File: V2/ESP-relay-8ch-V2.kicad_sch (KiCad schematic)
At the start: 143 parts, among them J1 +24VDC, J10 OUT8, J2 INPUTS, J3 OUT1, J4 OUT2, J5 OUT3, J6 OUT4, J7 OUT5, J8 OUT6, J9 OUT7, K1 G5PZ-1A, K2 G5PZ-1A, K3 G5PZ-1A, K4 G5PZ-1A, K5 G5PZ-1A, K6 G5PZ-1A, K7 G5PZ-1A, K8 G5PZ-1A, Q1 MMBT2222A/SOT-23-3, Q2 MMBT2222A/SOT-23-3, Q3 MMBT2222A/SOT-23-3, Q4 MMBT2222A/SOT-23-3, Q5 MMBT2222A/SOT-23-3, Q6 MMBT2222A/SOT-23-3, Q7 MMBT2222A/SOT-23-3, Q8 MMBT2222A/SOT-23-3, U1 SY8089A1AAC, U10 TX4138, U11 Olimex_ESP32-POE, U2 LTV-817S, U3 LTV-817S, U4 LTV-817S, U5 LTV-817S, U6 LTV-817S, U7 LTV-817S, U8 LTV-817S, U9 LTV-817S

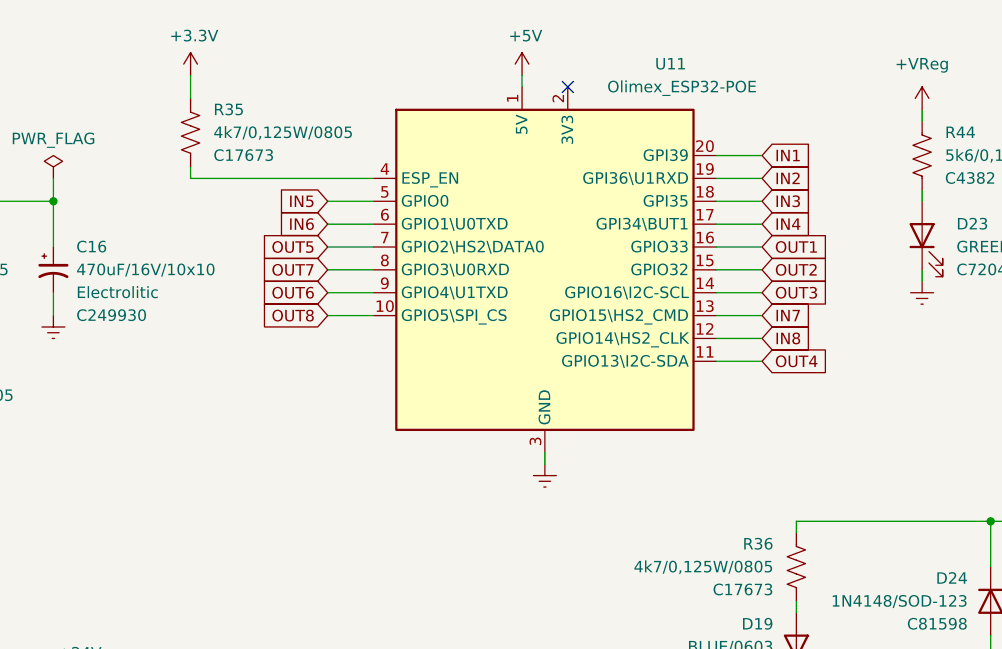
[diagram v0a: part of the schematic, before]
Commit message: Dev
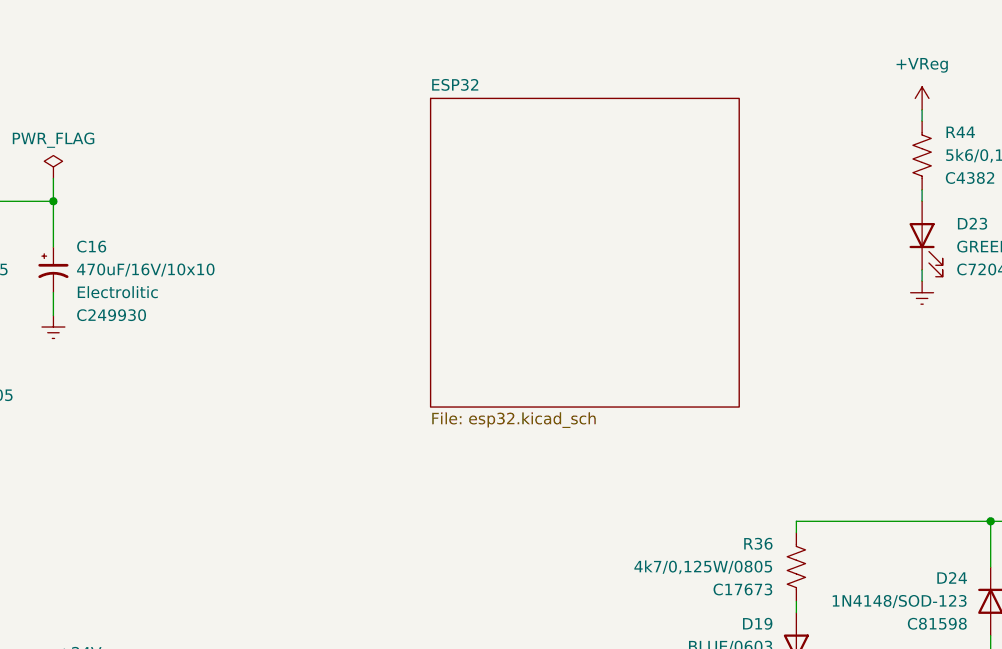
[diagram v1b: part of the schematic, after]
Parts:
- removed R35: 4k7/0,125W/0805, Tales:R_0805_2012Metric, symbol Device:R_US
- removed U11: Olimex_ESP32-POE, Tales:Olimex_ESP32-POE_Pads, symbol Tales:Olimex_ESP32-POE
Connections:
- no-connect marks 3 -> 2
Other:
- added sheet ESP32 (esp32.kicad_sch)
